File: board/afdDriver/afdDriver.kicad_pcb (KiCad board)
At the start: 2 copper layers, 45 parts, among them J1 SegmentEnables, J2 HighVoltageAC, J3 GND Pin #1, J4 GND Pin #2, U1 QTM3063T1, U2 QTM3063T1, U3 QTM3063T1, U4 QTM3063T1, U5 QTM3063T1, U6 QTM3063T1, U7 QTM3063T1, U8 QTM3063T1

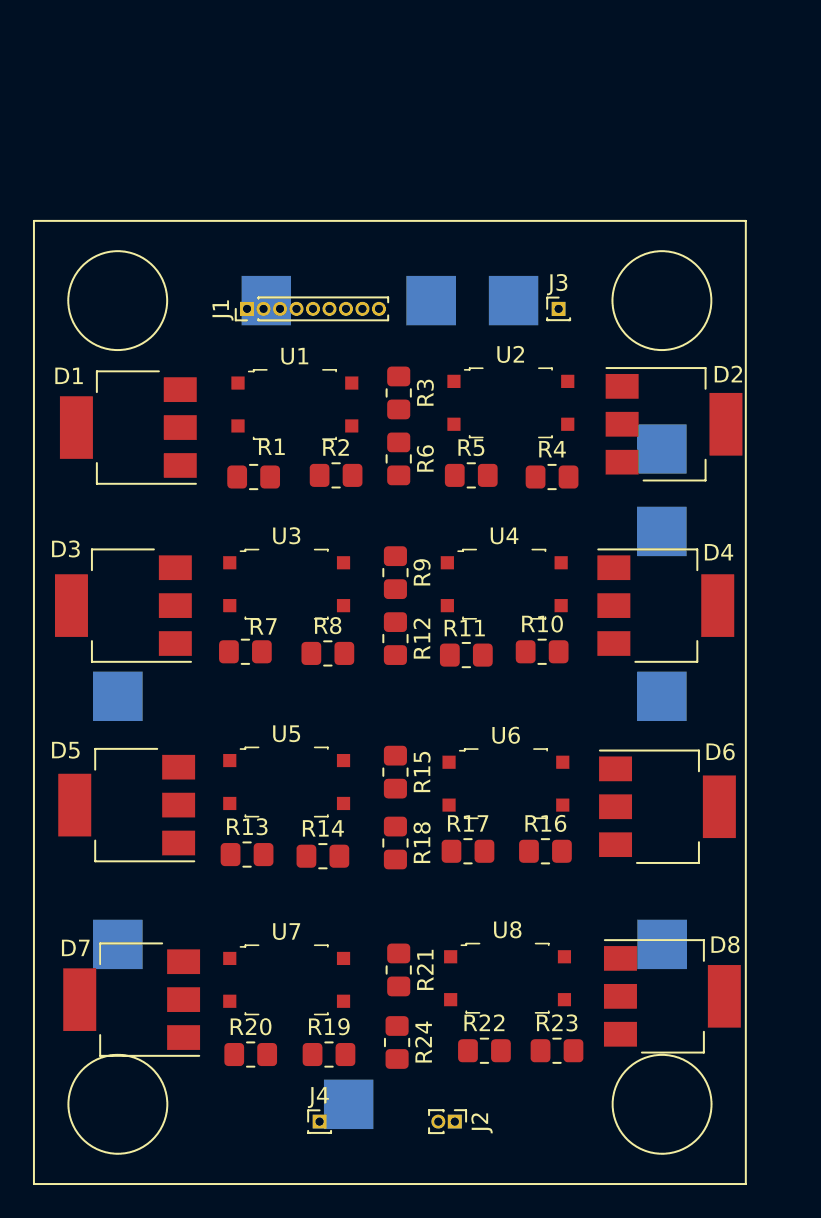
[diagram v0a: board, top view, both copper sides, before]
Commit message: Checkpoint. Starting layout.
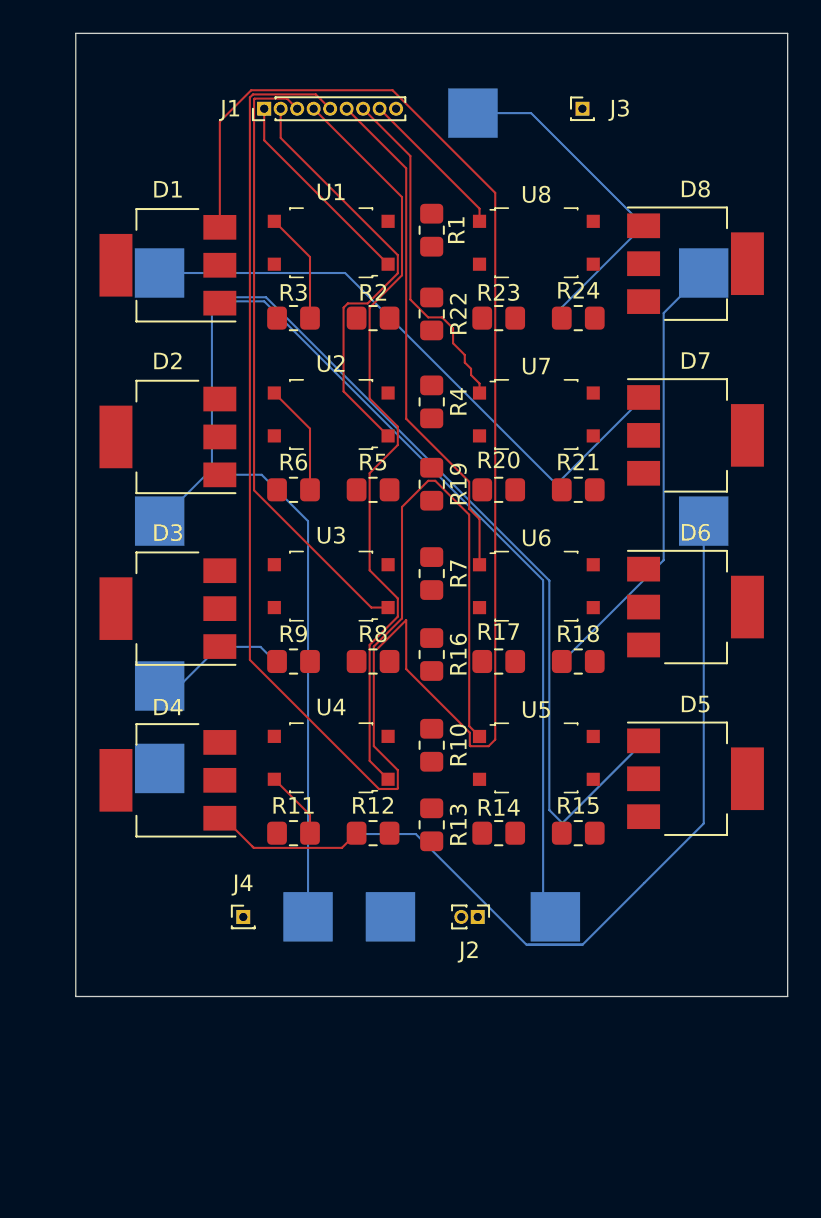
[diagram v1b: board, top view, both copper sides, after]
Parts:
- DS1: moved to B.Cu
- moved D7 48.4 mm to (117.6, 71.4), turned to 0 degrees
- moved R24 45.3 mm to (110.5, 64.3), turned to 0 degrees
- moved R22 44.8 mm to (101.6, 64.0), turned to 270 degrees
- moved U8 44.6 mm to (108.0, 59.7)
- moved R23 44.6 mm to (105.7, 64.3), turned to 180 degrees
- moved D8 44.5 mm to (117.6, 61.0)
- moved U7 37.5 mm to (108.0, 70.1)
- moved R20 37.4 mm to (105.7, 74.7), turned to 180 degrees
- moved R19 35.1 mm to (101.6, 74.3), turned to 270 degrees
- moved D5 34.5 mm to (117.6, 92.2), turned to 0 degrees
- moved D4 32.0 mm to (85.6, 92.3), turned to 180 degrees
- moved R21 31.1 mm to (110.5, 74.7), turned to 0 degrees
- moved D2 30.7 mm to (85.6, 71.5), turned to 180 degrees
- moved R1 18.5 mm to (101.6, 58.9), turned to 270 degrees
- moved R18 15.6 mm to (110.5, 85.1), turned to 0 degrees
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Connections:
- DS1 pad 5: Net-(DS1-Pad5) -> (no net)
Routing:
- net /EnbSegE: track 0.00 -> 89.3 mm
- net Net-(D1-Pad3): track 0.00 -> 79.8 mm
- net /SegE: track 0.00 -> 64.3 mm
- net /SegD: track 0.00 -> 57.9 mm
- net /SegA: track 0.00 -> 47.4 mm
- net /EnbSegD: track 0.00 -> 47.0 mm
- net /EnbSegC: track 0.00 -> 37.7 mm
- net /SegG: track 0.00 -> 37.4 mm
- net /EnbSegF: track 0.00 -> 31.0 mm
- net /SegB: track 0.00 -> 30.5 mm
- net /SegF: track 0.00 -> 27.1 mm
- net /EnbSegB: track 0.00 -> 26.0 mm
- net /SegH: track 0.00 -> 20.8 mm
- net /EnbSegG: track 0.00 -> 20.7 mm
- net /EnbSegA: track 0.00 -> 12.5 mm
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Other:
- board outline added: 43.2 x 58.4 mm
- copper layers 2 -> 4
- net class Default: clearance 0.2 -> 0.127; trace_width 0.25 -> 0.127; via_dia 0.8 -> 0.6; via_drill 0.4 -> 0.3
- rule trace_clearance: 0.2 -> 0.127
- rule trace_min: 0.2 -> 0.127
- rule via_min_size: 0.4 -> 0.6
